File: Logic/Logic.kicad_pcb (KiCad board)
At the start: 2 copper layers, 11 x 42 mm, 16 parts, among them J1 Conn_01x04_Pin

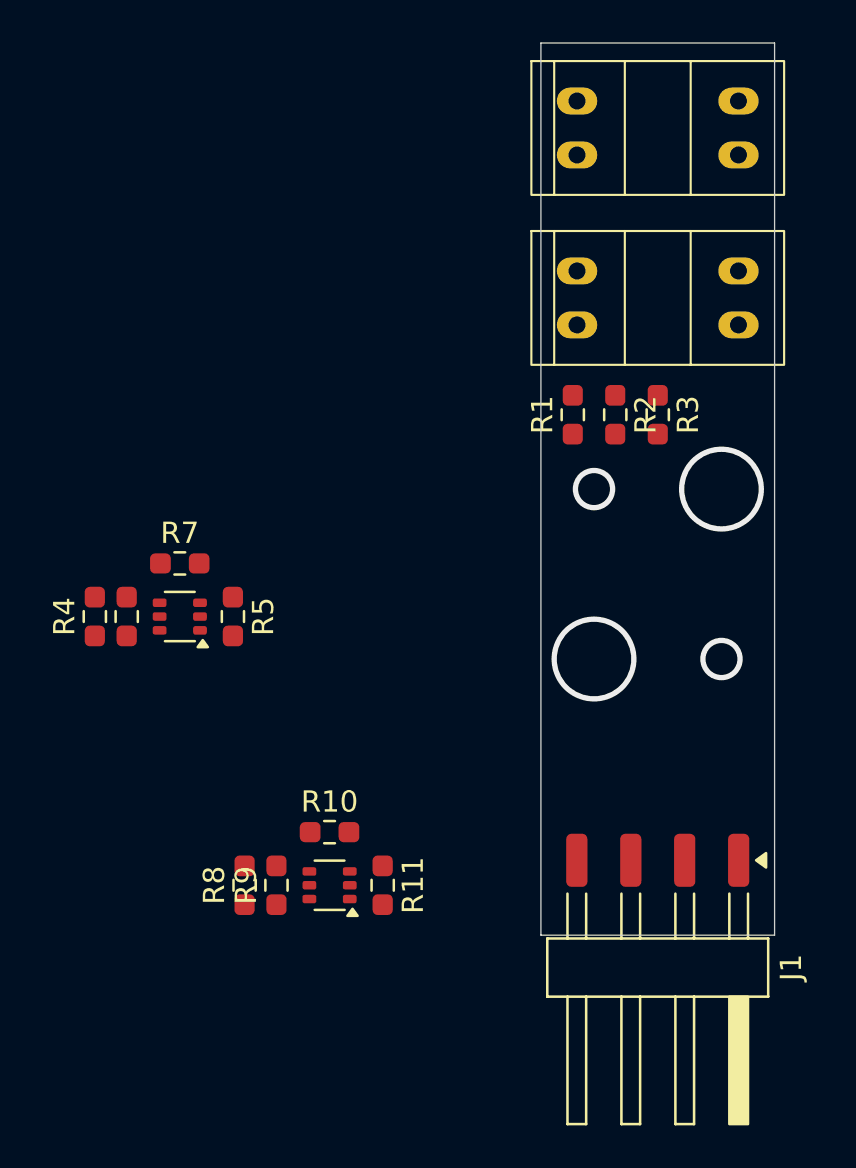
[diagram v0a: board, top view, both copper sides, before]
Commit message: user save
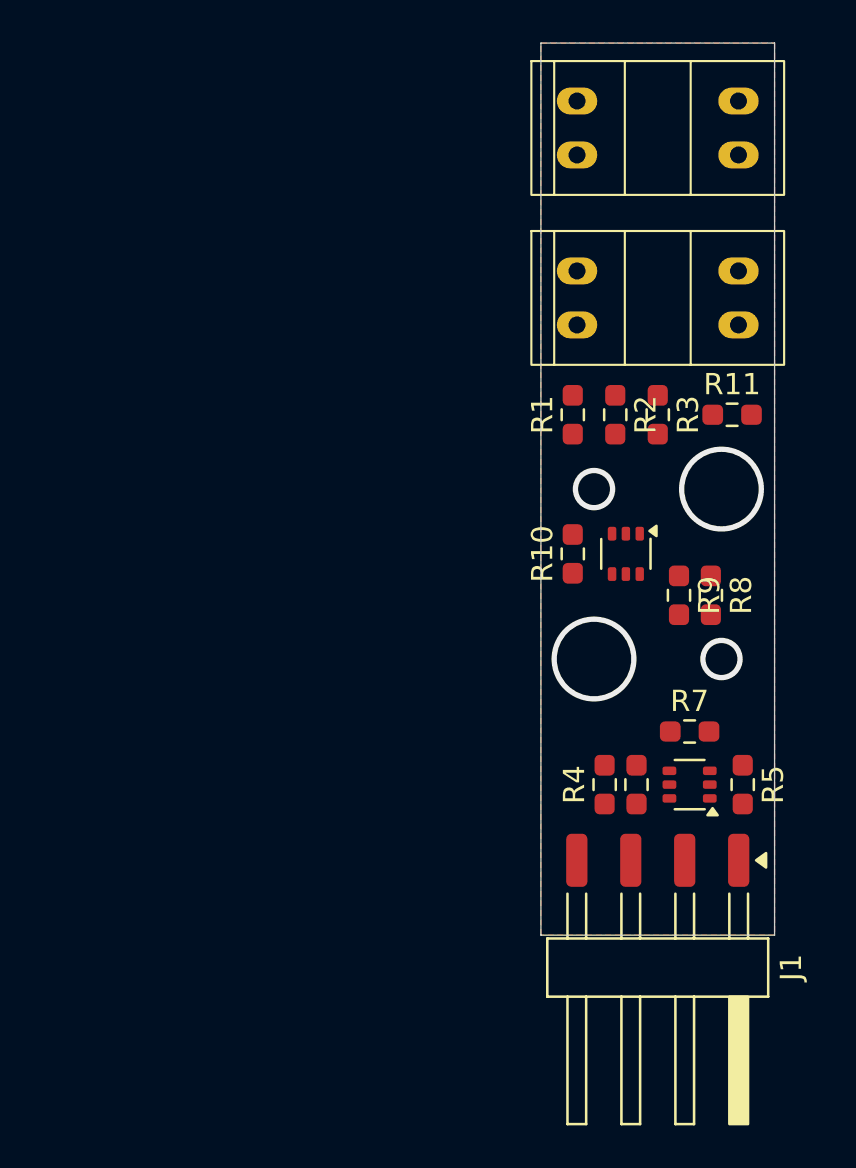
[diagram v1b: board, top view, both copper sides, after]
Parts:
- moved R11 27.6 mm to (152.0, 89.5), turned to 0 degrees
- moved R8 25.8 mm to (151.0, 98.0), turned to -90 degrees
- moved Q1 25.3 mm to (150.0, 106.9)
- moved R4 25.3 mm to (146.0, 106.9)
- moved R5 25.3 mm to (152.5, 106.9)
- moved R6 25.3 mm to (147.5, 106.9)
- moved R7 25.3 mm to (150.0, 104.4)
- moved R9 23.4 mm to (149.5, 98.0), turned to -90 degrees
- moved Q2 20.9 mm to (147.0, 96.0), turned to -90 degrees
- moved R10 17.4 mm to (144.5, 96.0), turned to 90 degrees
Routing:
- added copper zone on F.Cu, net GNDD

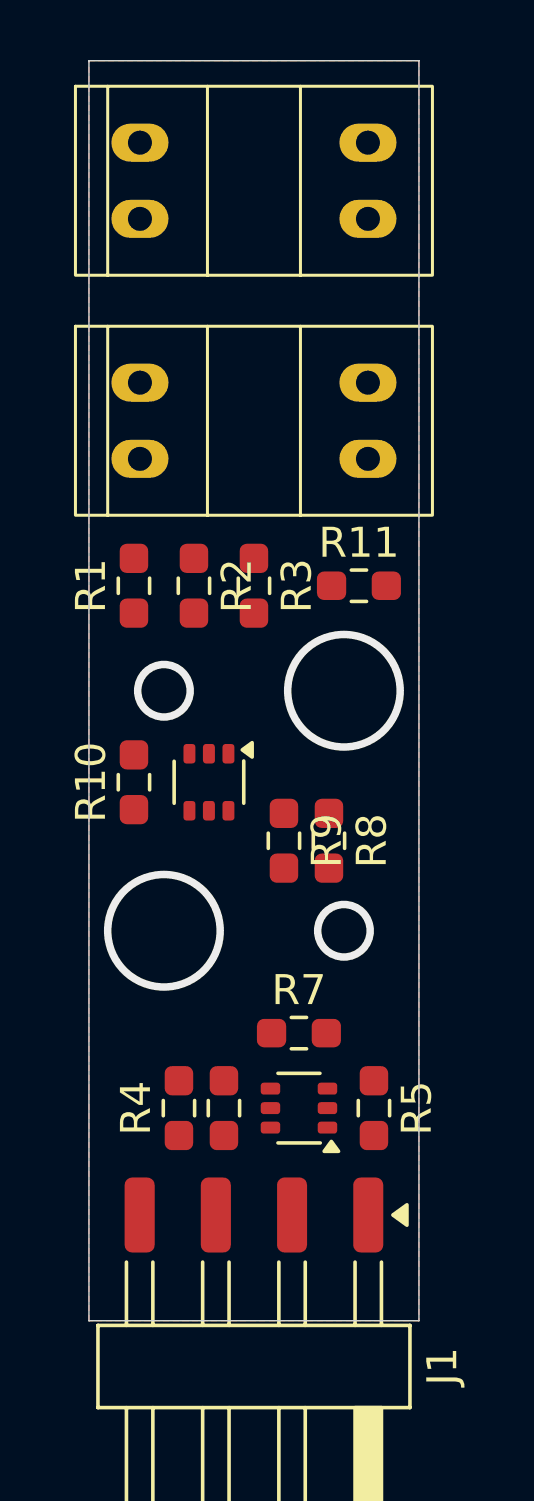
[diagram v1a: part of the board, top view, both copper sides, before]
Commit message: user saved
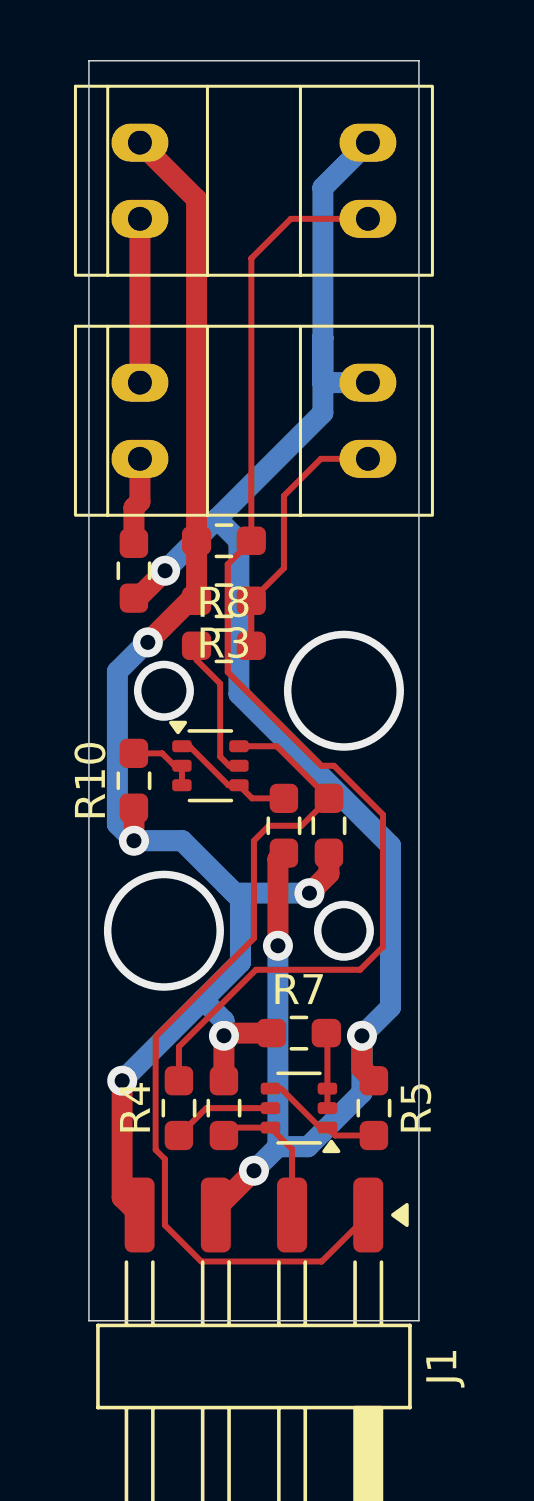
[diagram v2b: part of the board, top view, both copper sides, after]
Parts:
- moved R11 8.38 mm to (149.5, 97.5), turned to 90 degrees
- moved R8 7.38 mm to (147.5, 91.5), turned to 0 degrees
- moved R2 1.80 mm to (147.5, 88.0), turned to 180 degrees
- moved R9 1.58 mm to (151.0, 97.5)
- moved R3 1.12 mm to (147.5, 90.0), turned to 180 degrees
- moved Q2 0.55 mm to (147.1, 95.5), turned to 0 degrees
- moved R1 0.50 mm to (144.5, 89.0), turned to -90 degrees
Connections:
- R1 pad 1: VCC -> Net-(R1-Pad1)
- R1 pad 2: Net-(R1-Pad2) -> GNDD
- U1 pad 1: Net-(U1-Pad1) -> VCC
- U1 pad 2: GNDD -> Net-(U1-Pad2)
- U2 pad 1: Net-(R1-Pad2) -> Net-(U1-Pad2)
- U2 pad 2: Net-(U1-Pad1) -> Net-(R1-Pad1)
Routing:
- net GNDD: track 0.00 -> 61.6 mm, vias 0 -> 4
- net VCC: track 0.00 -> 52.5 mm, vias 0 -> 5
- net Net-(R2-Pad1): track 0.00 -> 39.4 mm
- net Net-(J1-Pin_1): track 0.00 -> 29.0 mm
- net Net-(R3-Pad1): track 0.00 -> 8.76 mm
- net Net-(U1-Pad2): track 0.00 -> 5.46 mm
- net Net-(J1-Pin_2): track 0.00 -> 4.87 mm
- net Net-(Q2-Pad5): track 0.00 -> 4.78 mm
- net Net-(Q2-Pad1): track 0.00 -> 4.12 mm
- net Net-(Q1-Pad1): track 0.00 -> 4.10 mm
- net Net-(Q1-Pad5): track 0.00 -> 3.43 mm
- net Net-(R1-Pad1): track 0.00 -> 2.90 mm
- net Net-(Q1-Pad2): track 0.00 -> 2.52 mm
- net Net-(Q2-Pad2): track 0.00 -> 2.42 mm
- removed copper zone on F.Cu, net GNDD
